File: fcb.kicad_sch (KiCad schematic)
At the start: 21 parts, among them U1 TPS5430DDA, U2 AMS1117-3.3, U3 DL-RTS4432, U4 LSM6DS3, U5 STM32F411CEUx

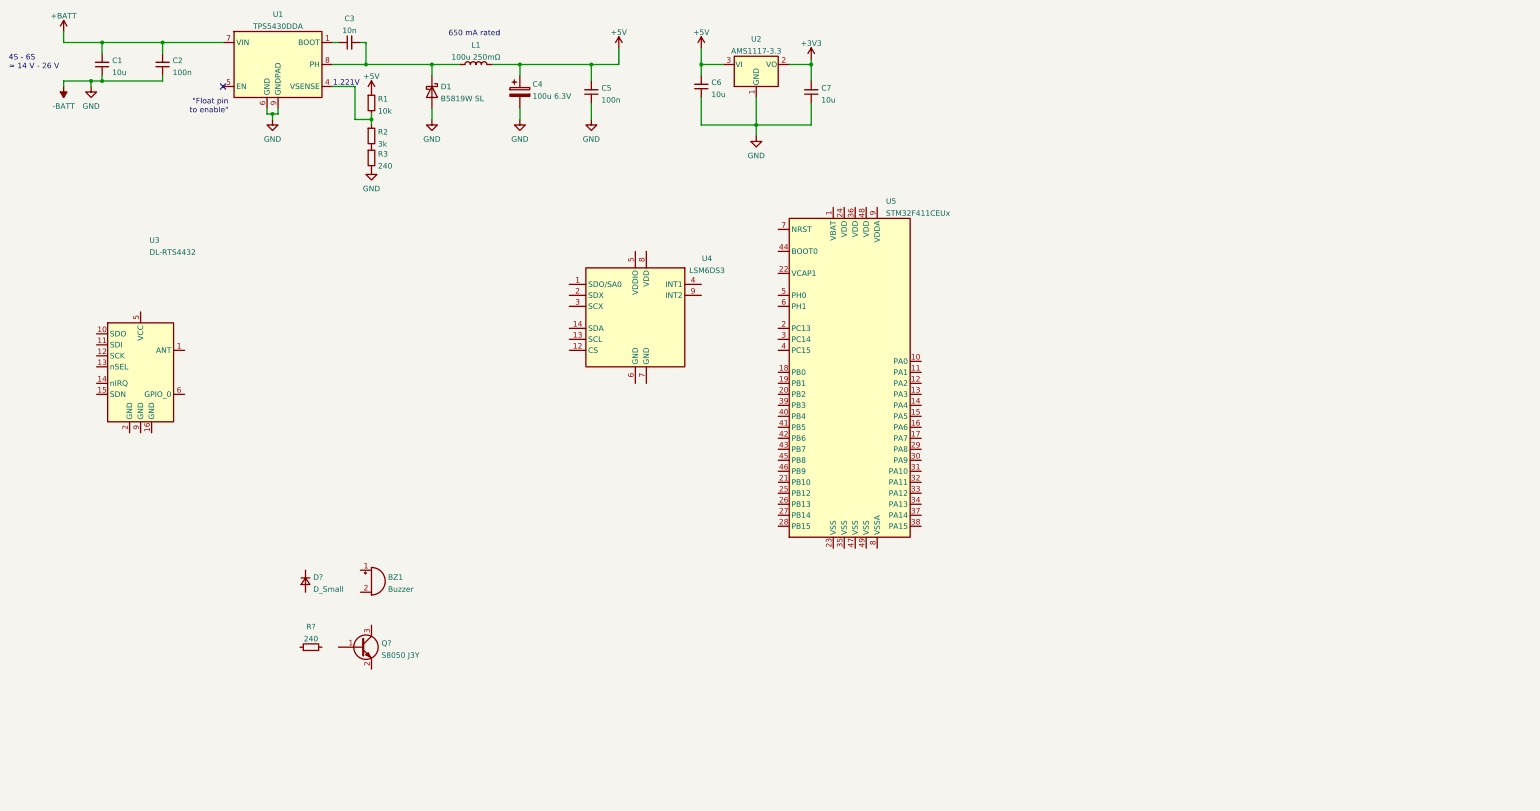
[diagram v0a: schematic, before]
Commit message: alku säätöä.
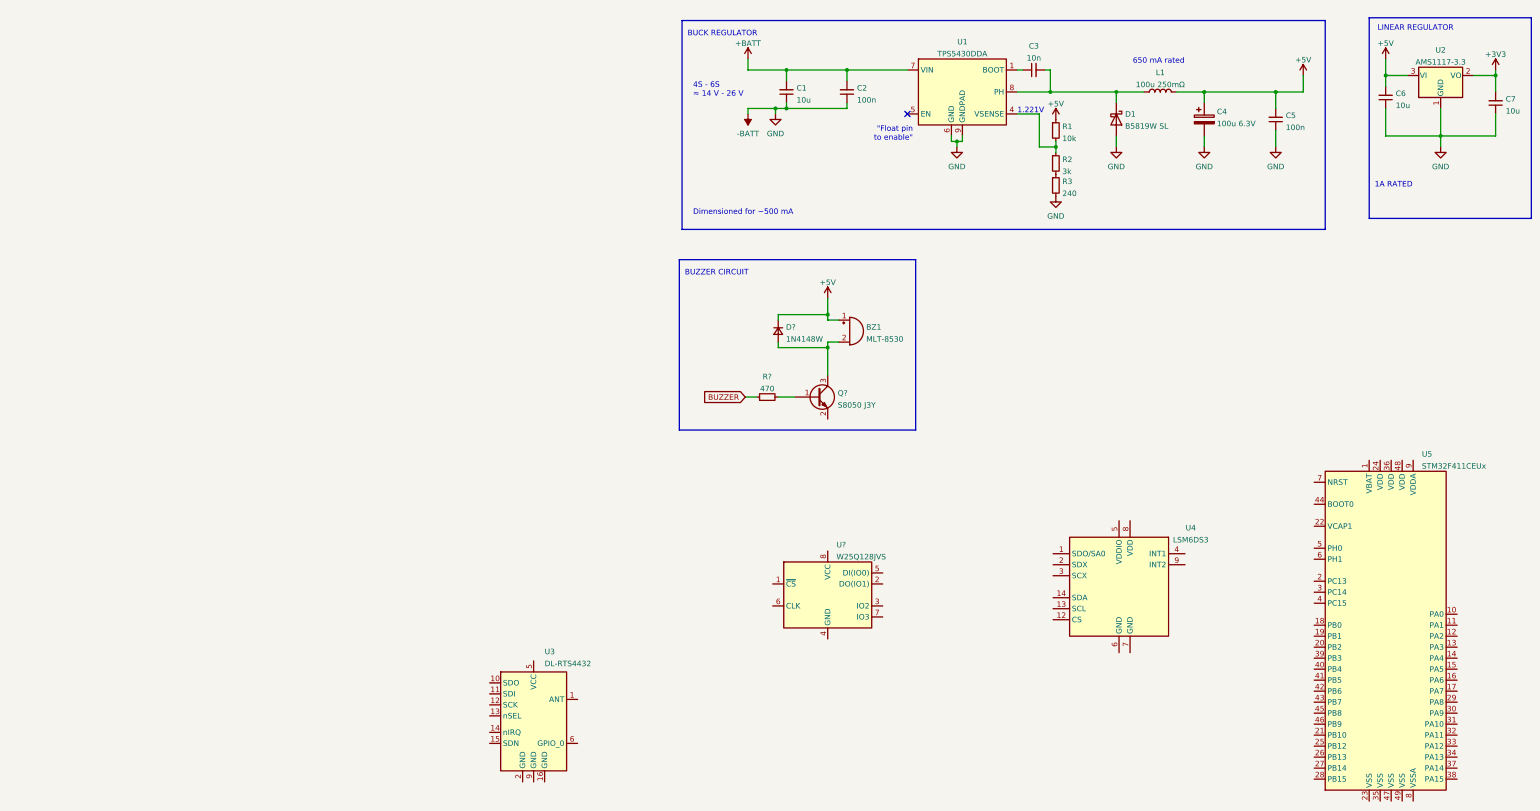
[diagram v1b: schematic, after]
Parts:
- added U?: W25Q128JVS, Package_SO:SOIC-8_5.23x5.23mm_P1.27mm, symbol Memory_Flash:W25Q128JVS
- BZ1: value Buzzer -> MLT-8530; LCSC (none) -> C94599
- D?: value D_Small -> 1N4148W; footprint (none) -> Diode_SMD:D_SOD-123; LCSC (none) -> C81598
- R?: value 240 -> 470; LCSC C23350 -> C23179
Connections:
- net +5V: now also BZ1.1 (-), D?.1 (K)
- net at Q?.1 (B): now also R?.2
- net at Q?.3 (C): now also BZ1.2 (+), D?.2 (A)
- net BUZZER: now reaches R?.1
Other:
- note added: "1A RATED"
- note added: "BUCK REGULATOR"
- note added: "BUZZER CIRCUIT"
- note added: "Dimensioned for ~500 mA"
- note added: "LINEAR REGULATOR"
- moved on the sheet: BZ1, C1, C2, C3, C4, C5, C6, C7, D1, D?, L1, Q?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
